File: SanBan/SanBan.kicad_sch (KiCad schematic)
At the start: 33 parts, among them IC1 AP64500SP-13, J1 Conn_01x12_Pin, J10 Conn_01x03_Pin, J11 Conn_01x03_Pin, J12 Conn_01x03_Pin, J13 Conn_01x03_Pin, J14 Conn_01x02, J2 Conn_01x12_Pin, J3 Conn_01x09_Pin, J4 Conn_01x02, J5 Conn_02x03_Top_Bottom, J6 Conn_01x03_Pin, J7 Conn_01x03_Pin, J8 Conn_01x03_Pin, J9 Conn_01x03_Pin, SW1 SW_Push_Dual, U1 ATmega328PB-A, Y1 16M

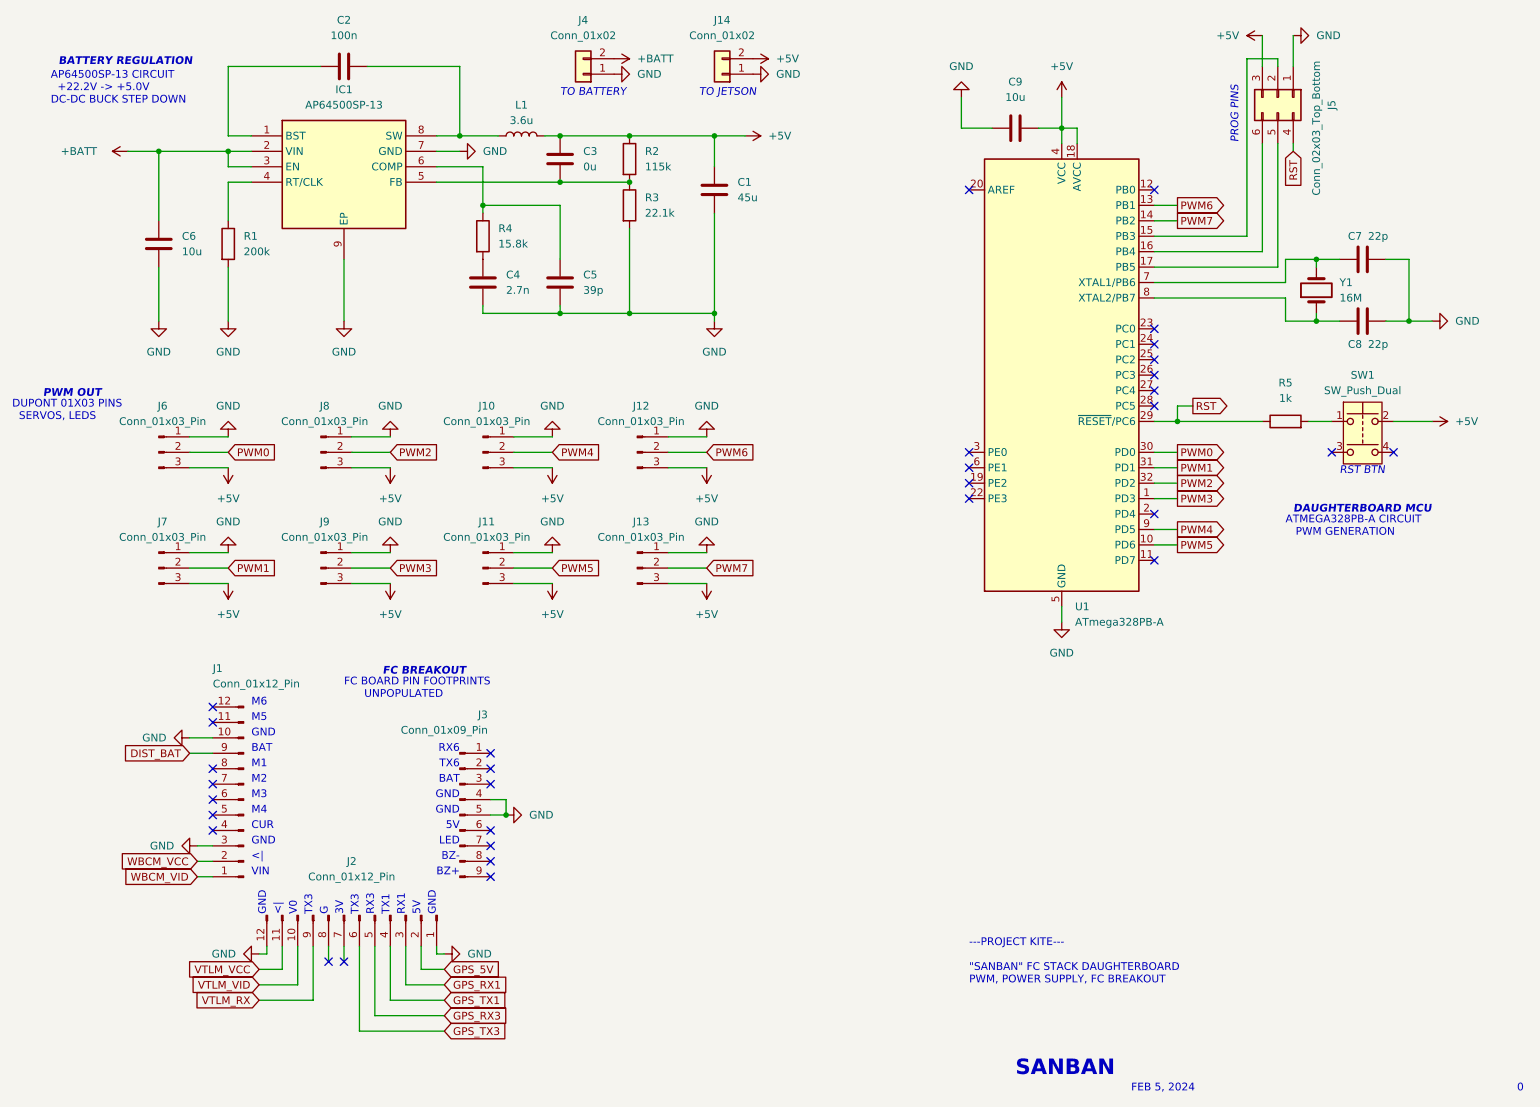
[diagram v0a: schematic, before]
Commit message: Started PCB layout
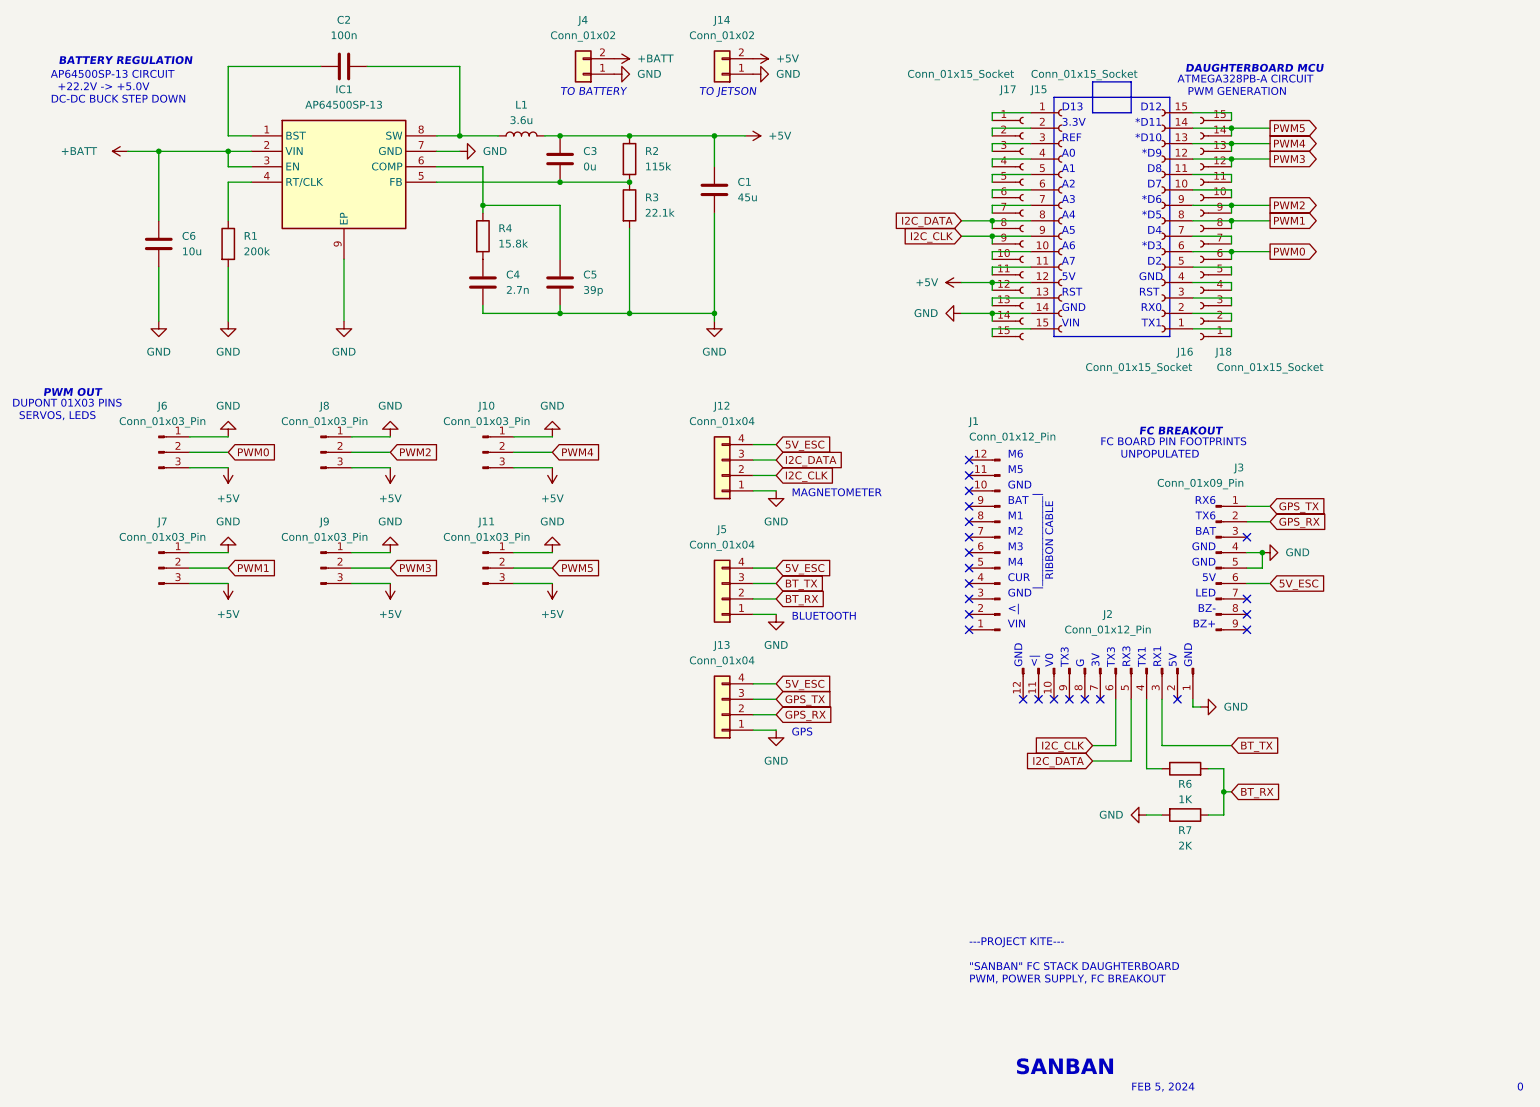
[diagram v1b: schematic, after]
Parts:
- removed C7, C8: 22p, symbol Device:C
- removed C9: 10u, symbol Device:C
- removed J12, J13: Conn_01x03_Pin, symbol Connector:Conn_01x03_Pin
- removed J5: Conn_02x03_Top_Bottom, symbol Connector_Generic:Conn_02x03_Top_Bottom
- removed R5: 1k, symbol Device:R
- removed SW1: SW_Push_Dual, symbol Switch:SW_Push_Dual
- removed U1: ATmega328PB-A, Package_QFP:TQFP-32_7x7mm_P0.8mm, symbol MCU_Microchip_ATmega:ATmega328PB-A
- removed Y1: 16M, symbol Device:Crystal
- added J12, J13, J5: Conn_01x04, Connector_JST:JST_EH_B4B-EH-A_1x04_P2.50mm_Vertical, symbol Connector_Generic:Conn_01x04
- added J15, J16, J17, J18: Conn_01x15_Socket, Connector_PinSocket_2.54mm:PinSocket_1x15_P2.54mm_Vertical, symbol Connector:Conn_01x15_Socket
- added R6: 1K, Capacitor_SMD:C_0805_2012Metric_Pad1.18x1.45mm_HandSolder, symbol Device:R
- added R7: 2K, Capacitor_SMD:C_0805_2012Metric_Pad1.18x1.45mm_HandSolder, symbol Device:R
- C1, C2, C3, C4, C5, C6, R1, R2, R3, R4: footprint (none) -> Capacitor_SMD:C_0805_2012Metric_Pad1.18x1.45mm_HandSolder
- IC1: footprint SOIC127P600X163-9N -> SanBanLibrary:SOIC127P600X163-9N
- J1, J2: footprint (none) -> Connector_PinSocket_2.54mm:PinSocket_1x12_P2.54mm_Vertical
- J10, J11, J6, J7, J8, J9: footprint (none) -> Connector_PinHeader_2.54mm:PinHeader_1x03_P2.54mm_Horizontal
- J14: footprint (none) -> Connector_JST:JST_EH_B2B-EH-A_1x02_P2.50mm_Vertical
- J3: footprint (none) -> Connector_PinSocket_2.00mm:PinSocket_1x09_P2.00mm_Vertical
- J4: footprint (none) -> Connector_Wire:SolderWire-0.127sqmm_1x02_P3.7mm_D0.48mm_OD1mm
- L1: footprint (none) -> Inductor_SMD:L_TDK_VLS6045EX_VLS6045AF
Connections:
- net +5V: now also J15.12 (Pin_12), J17.12 (Pin_12)
- net GND: now also J12.1 (Pin_1), J13.1 (Pin_1), J15.14 (Pin_14), J17.14 (Pin_14), J5.1 (Pin_1), R7.2; no longer J1.10 (Pin_10), J1.3 (Pin_3), J2.12 (Pin_12)
- net PWM0: now also J16.6 (Pin_6), J18.6 (Pin_6)
- net PWM1: now also J16.8 (Pin_8), J18.8 (Pin_8)
- net PWM2: now also J16.9 (Pin_9), J18.9 (Pin_9)
- net PWM3: now also J16.12 (Pin_12), J18.12 (Pin_12)
- net PWM4: now also J16.13 (Pin_13), J18.13 (Pin_13)
- net PWM5: now also J16.14 (Pin_14), J18.14 (Pin_14)
- net GPS_TX: now reaches J3.1 (Pin_1)
- net GPS_TX: now also J13.3 (Pin_3)
- net GPS_RX: now reaches J3.2 (Pin_2)
- net GPS_RX: now also J13.2 (Pin_2)
- net 5V_ESC: now reaches J3.6 (Pin_6)
- net 5V_ESC: now also J12.4 (Pin_4), J13.4 (Pin_4), J5.4 (Pin_4)
- net DIST_BAT: no longer names the net of J1.9 (Pin_9)
- net GPS_5V: no longer names the net of J2.2 (Pin_2)
- net GPS_RX1 renamed BT_TX
- net BT_TX: now also J5.3 (Pin_3)
- net GPS_RX3 renamed I2C_DATA
- net I2C_DATA: now also J12.3 (Pin_3), J15.8 (Pin_8), J17.8 (Pin_8)
- net GPS_TX1: no longer names the net of J2.4 (Pin_4)
- net GPS_TX1: now also R6.1
- net GPS_TX3 renamed I2C_CLK
- net I2C_CLK: now also J12.2 (Pin_2), J15.9 (Pin_9), J17.9 (Pin_9)
- net VTLM_RX: no longer names the net of J2.9 (Pin_9)
- net VTLM_VCC: no longer names the net of J2.11 (Pin_11)
- net VTLM_VID: no longer names the net of J2.10 (Pin_10)
- net WBCM_VCC: no longer names the net of J1.2 (Pin_2)
- net WBCM_VID: no longer names the net of J1.1 (Pin_1)
- new net: J15.1 (Pin_1), J17.1 (Pin_1)
- new net: J15.10 (Pin_10), J17.10 (Pin_10)
- new net: J15.11 (Pin_11), J17.11 (Pin_11)
- new net: J15.13 (Pin_13), J17.13 (Pin_13)
- new net: J15.15 (Pin_15), J17.15 (Pin_15)
- new net: J15.2 (Pin_2), J17.2 (Pin_2)
- new net: J15.3 (Pin_3), J17.3 (Pin_3)
- new net: J15.4 (Pin_4), J17.4 (Pin_4)
- new net: J15.5 (Pin_5), J17.5 (Pin_5)
- new net: J15.6 (Pin_6), J17.6 (Pin_6)
- new net: J15.7 (Pin_7), J17.7 (Pin_7)
- new net: J16.1 (Pin_1), J18.1 (Pin_1)
- new net: J16.10 (Pin_10), J18.10 (Pin_10)
- new net: J16.11 (Pin_11), J18.11 (Pin_11)
- new net: J16.15 (Pin_15), J18.15 (Pin_15)
- new net: J16.2 (Pin_2), J18.2 (Pin_2)
- new net: J16.3 (Pin_3), J18.3 (Pin_3)
- new net: J16.4 (Pin_4), J18.4 (Pin_4)
- new net: J16.5 (Pin_5), J18.5 (Pin_5)
- new net: J16.7 (Pin_7), J18.7 (Pin_7)
- new net BT_RX: J5.2 (Pin_2), R6.2, R7.1
- no-connect marks 32 -> 23
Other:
- note added: "*D10"
- note added: "*D11"
- note added: "*D3"
- note added: "*D5"
- note added: "*D6"
- note added: "*D9"
- note added: "3.3V"
- note added: "A0"
- note added: "A1"
- note added: "A2"
- note added: "A3"
- note added: "A4"
- note added: "A5"
- note added: "A6"
- note added: "A7"
- note added: "BLUETOOTH"
- note added: "D12"
- note added: "D13"
- note added: "D2"
- note added: "D4"
- note added: "D7"
- note added: "D8"
- note added: "GPS"
- note added: "MAGNETOMETER"
- note added: "REF"
- note added: "RST"
- note added: "RX0"
- note added: "|_________________| RIBBON CABLE"
- note removed: "PROG PINS"
- note removed: "RST BTN"
- moved on the sheet: J1, J2, J3

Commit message: SanBan Rev 1.0
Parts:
- J1, J2: footprint Connector_PinSocket_2.54mm:PinSocket_1x12_P2.54mm_Vertical -> Connector_PinSocket_2.00mm:PinSocket_1x12_P2.00mm_Vertical
- J10, J11, J6, J7, J8, J9: footprint Connector_PinHeader_2.54mm:PinHeader_1x03_P2.54mm_Horizontal -> Connector_PinHeader_2.54mm:PinHeader_1x03_P2.54mm_Vertical
- J3: footprint Connector_PinSocket_2.00mm:PinSocket_1x09_P2.00mm_Vertical -> Connector_PinSocket_2.54mm:PinSocket_1x09_P2.54mm_Vertical
- J4: footprint Connector_Wire:SolderWire-0.127sqmm_1x02_P3.7mm_D0.48mm_OD1mm -> Connector_PinHeader_2.54mm:PinHeader_1x02_P2.54mm_Horizontal
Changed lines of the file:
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@@
       (effects (font (size 1.27 1.27)))
     )
-    (property "Footprint" "Connector_PinHeader_2.54mm:PinHeader_1x03_P2.54mm_Horizontal" (at 72.39 88.9 0)
+    (property "Footprint" "Connector_PinHeader_2.54mm:PinHeader_1x03_P2.54mm_Vertical" (at 72.39 88.9 0)
       (effects (font (size 1.27 1.27)) hide)
     )
@@
       (effects (font (size 1.27 1.27)))
     )
-    (property "Footprint" "Connector_PinHeader_2.54mm:PinHeader_1x03_P2.54mm_Horizontal" (at 72.39 107.95 0)
+    (property "Footprint" "Connector_PinHeader_2.54mm:PinHeader_1x03_P2.54mm_Vertical" (at 72.39 107.95 0)
       (effects (font (size 1.27 1.27)) hide)
     )
@@
       (effects (font (size 1.27 1.27)) (justify right))
     )
-    (property "Footprint" "Connector_PinSocket_2.54mm:PinSocket_1x12_P2.54mm_Vertical" (at 184.15 105.41 0)
+    (property "Footprint" "Connector_PinSocket_2.00mm:PinSocket_1x12_P2.00mm_Vertical" (at 184.15 105.41 0)
       (effects (font (size 1.27 1.27)) hide)
     )
@@
       (effects (font (size 1.27 1.27)))
     )
-    (property "Footprint" "Connector_PinHeader_2.54mm:PinHeader_1x03_P2.54mm_Horizontal" (at 45.72 107.95 0)
+    (property "Footprint" "Connector_PinHeader_2.54mm:PinHeader_1x03_P2.54mm_Vertical" (at 45.72 107.95 0)
       (effects (font (size 1.27 1.27)) hide)
     )
@@
       (effects (font (size 1.27 1.27)))
     )
-    (property "Footprint" "Connector_PinSocket_2.00mm:PinSocket_1x09_P2.00mm_Vertical" (at 219.71 107.95 0)
+    (property "Footprint" "Connector_PinSocket_2.54mm:PinSocket_1x09_P2.54mm_Vertical" (at 219.71 107.95 0)
       (effects (font (size 1.27 1.27)) hide)
     )
@@
       (effects (font (size 1.27 1.27)))
     )
-    (property "Footprint" "Connector_PinHeader_2.54mm:PinHeader_1x03_P2.54mm_Horizontal" (at 45.72 88.9 0)
+    (property "Footprint" "Connector_PinHeader_2.54mm:PinHeader_1x03_P2.54mm_Vertical" (at 45.72 88.9 0)
       (effects (font (size 1.27 1.27)) hide)
     )
@@
       (effects (font (size 1.27 1.27)))
     )
-    (property "Footprint" "Connector_PinSocket_2.54mm:PinSocket_1x12_P2.54mm_Vertical" (at 203.2 124.46 0)
+    (property "Footprint" "Connector_PinSocket_2.00mm:PinSocket_1x12_P2.00mm_Vertical" (at 203.2 124.46 0)
       (effects (font (size 1.27 1.27)) hide)
     )
@@
       (effects (font (size 1.27 1.27)))
     )
-    (property "Footprint" "Connector_PinHeader_2.54mm:PinHeader_1x03_P2.54mm_Horizontal" (at 99.06 88.9 0)
+    (property "Footprint" "Connector_PinHeader_2.54mm:PinHeader_1x03_P2.54mm_Vertical" (at 99.06 88.9 0)
       (effects (font (size 1.27 1.27)) hide)
     )
@@
       (effects (font (size 1.27 1.27)))
     )
-    (property "Footprint" "Connector_PinHeader_2.54mm:PinHeader_1x03_P2.54mm_Horizontal" (at 99.06 107.95 0)
+    (property "Footprint" "Connector_PinHeader_2.54mm:PinHeader_1x03_P2.54mm_Vertical" (at 99.06 107.95 0)
       (effects (font (size 1.27 1.27)) hide)
     )
@@
       (effects (font (size 1.27 1.27)))
     )
-    (property "Footprint" "Connector_Wire:SolderWire-0.127sqmm_1x02_P3.7mm_D0.48mm_OD1mm" (at 115.57 26.67 0)
-      (effects (font (size 1.27 1.27)) hide)
-    )
+    (property "Footprint" "Connector_PinHeader_2.54mm:PinHeader_1x02_P2.54mm_Horizontal" (at 115.57 26.67 0)
+      (effects (font (size 1.27 1.27)) hide)
+    )
